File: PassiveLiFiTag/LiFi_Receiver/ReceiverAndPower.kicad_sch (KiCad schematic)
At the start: 10 parts, among them U1 TS881ILT, U3 BQ25570RGRR

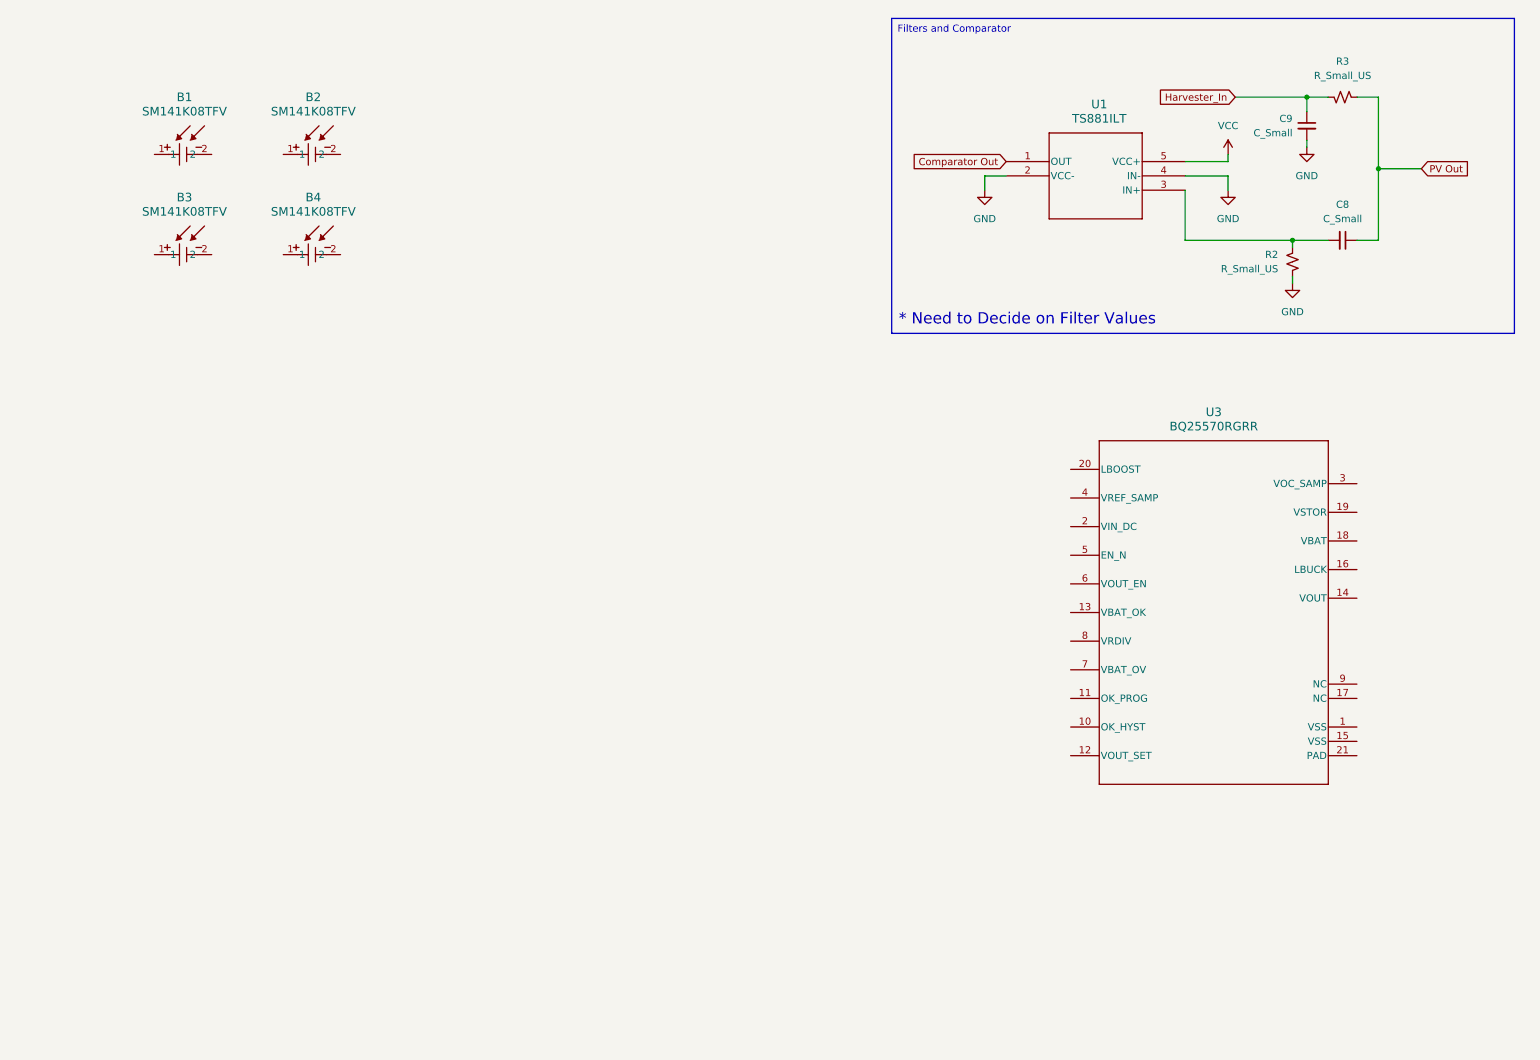
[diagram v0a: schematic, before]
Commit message: Continuing to update Hardware Design
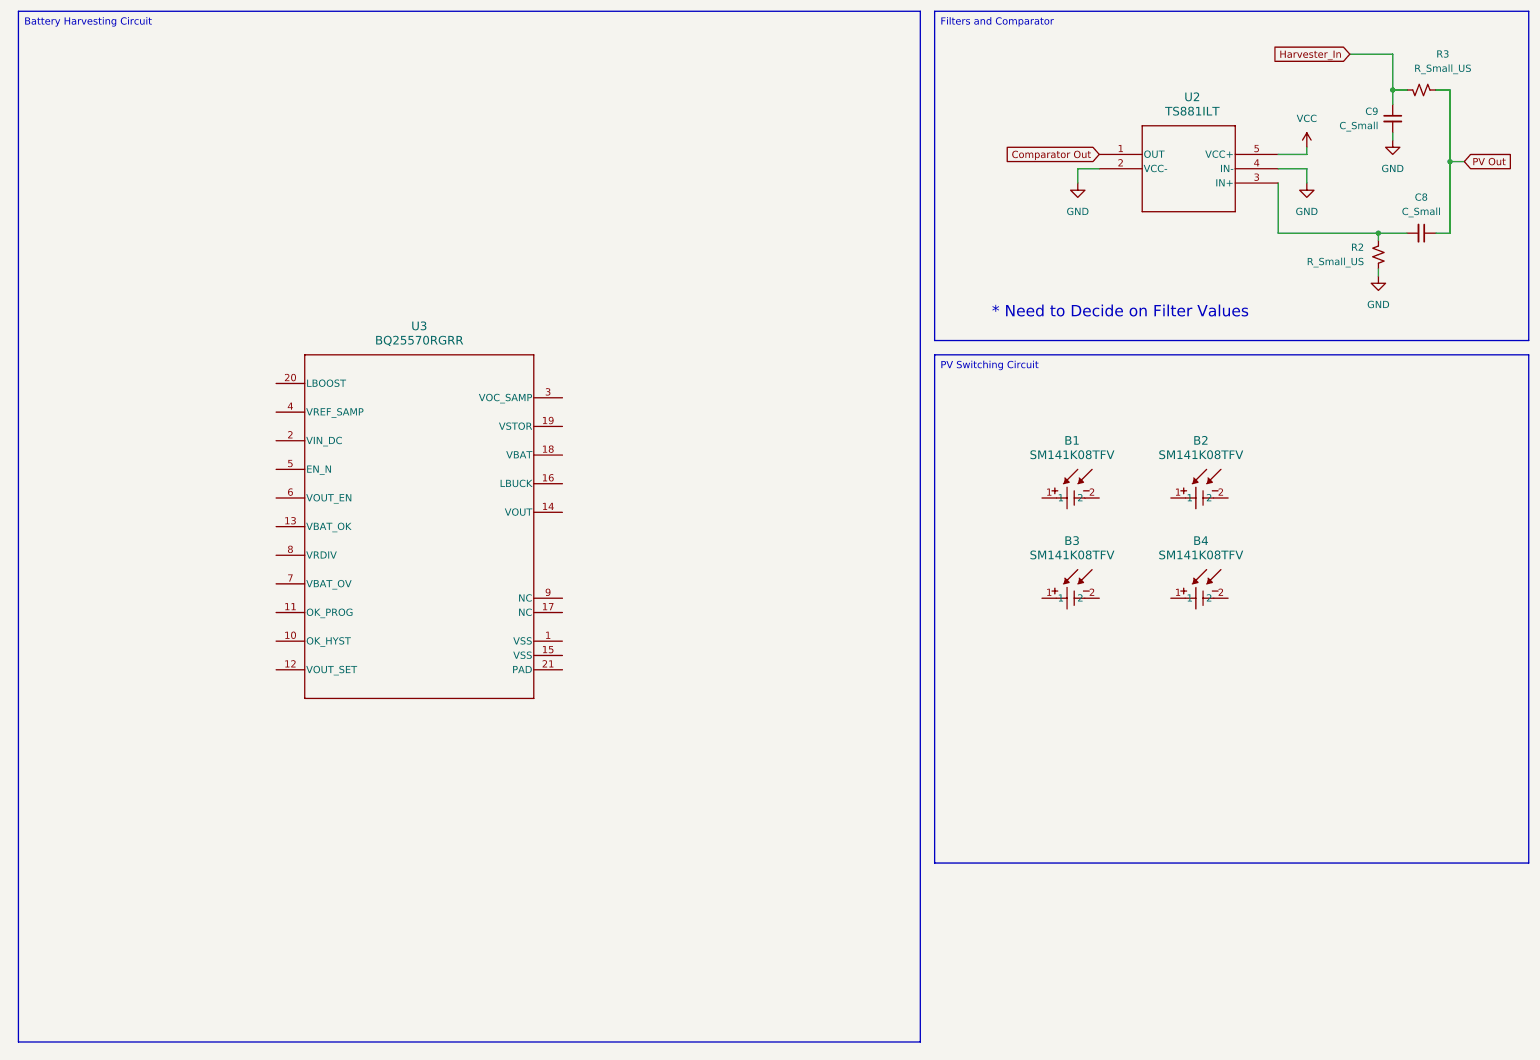
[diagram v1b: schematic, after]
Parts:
- renumbered U1 to U2
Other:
- moved on the sheet: B1, B2, B3, B4, C8, C9, R2, R3, U2, U3

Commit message: updating changes
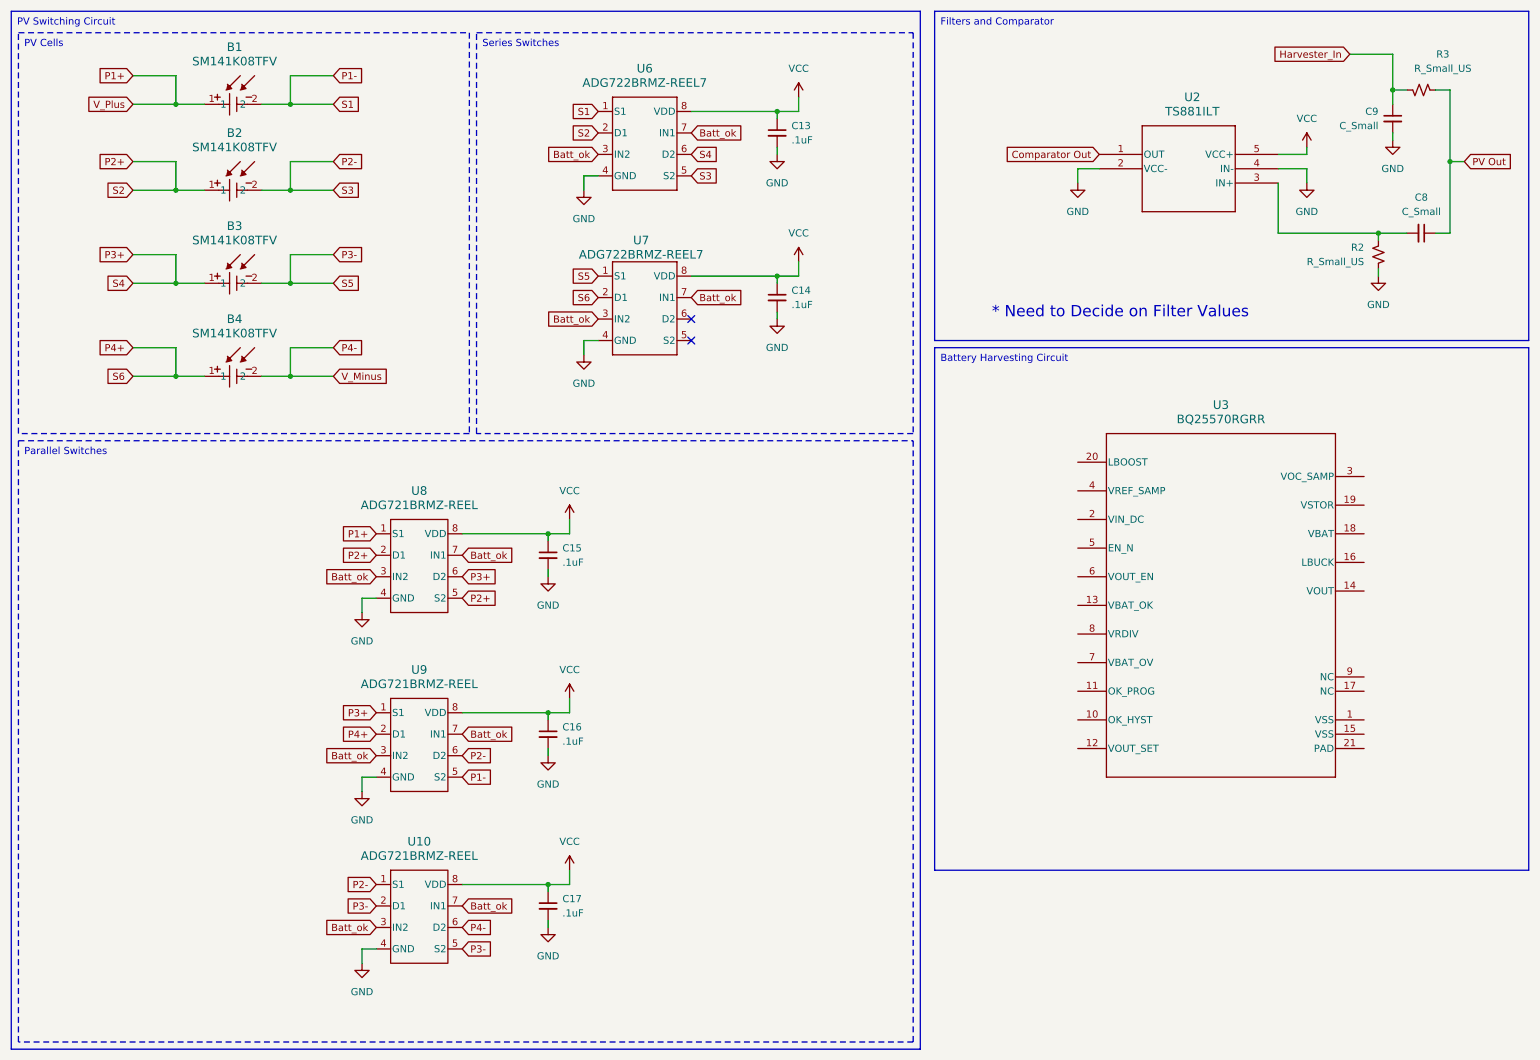
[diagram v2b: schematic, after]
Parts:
- added C13, C14, C15, C16, C17: .1uF, symbol Device:C_Small
- added U10, U8, U9: ADG721BRMZ-REEL, RM_8_ADI, symbol LiFi_Receiver:ADG721BRMZ-REEL
- added U6, U7: ADG722BRMZ-REEL7, RM_8_ADI, symbol LiFi_Receiver:ADG722BRMZ-REEL7
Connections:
- net GND: now also C13.2, C14.2, C15.2, C16.2, C17.2, U10.4 (GND), U6.4 (GND), U7.4 (GND), U8.4 (GND), U9.4 (GND)
- net VCC: now also C13.1, C14.1, C15.1, C16.1, C17.1, U10.8 (VDD), U6.8 (VDD), U7.8 (VDD), U8.8 (VDD), U9.8 (VDD)
- net P2+: now reaches B2.1
- net P2+: now also U6.2 (D1), U8.2 (D1), U8.5 (S2)
- net P2-: now reaches B2.2
- net P2-: now also U10.1 (S1), U6.5 (S2), U9.6 (D2)
- net P3+: now reaches B3.1
- net P3+: now also U6.6 (D2), U8.6 (D2), U9.1 (S1)
- net P3-: now reaches B3.2
- net P3-: now also U10.2 (D1), U10.5 (S2), U7.1 (S1)
- net P1+: now reaches B1.1
- net P1+: now also U8.1 (S1)
- net P1-: now reaches B1.2
- net P1-: now also U6.1 (S1), U9.5 (S2)
- net P4+: now reaches B4.1
- net P4+: now also U7.2 (D1), U9.2 (D1)
- net P4-: now reaches B4.2
- net P4-: now also U10.6 (D2)
- new net Batt_ok: U10.3 (IN2), U10.7 (IN1), U6.3 (IN2), U6.7 (IN1), U7.3 (IN2), U7.7 (IN1), U8.3 (IN2), U8.7 (IN1), U9.3 (IN2), U9.7 (IN1)
- no-connect marks 0 -> 2
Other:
- moved on the sheet: B1, B2, B3, B4, U3

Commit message: added Updates
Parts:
- C13, C14, C15, C16, C17: footprint (none) -> Capacitor_SMD:C_01005_0402Metric
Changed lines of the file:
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@@
       (effects (font (size 1.27 1.27)) (justify right))
     )
-    (property "Footprint" "" (at 149.86 34.29 0)
+    (property "Footprint" "Capacitor_SMD:C_01005_0402Metric" (at 149.86 34.29 0)
       (effects (font (size 1.27 1.27)) hide)
     )
@@
       (effects (font (size 1.27 1.27)) (justify right))
     )
-    (property "Footprint" "" (at 109.22 109.22 0)
+    (property "Footprint" "Capacitor_SMD:C_01005_0402Metric" (at 109.22 109.22 0)
       (effects (font (size 1.27 1.27)) hide)
     )
@@
       (effects (font (size 1.27 1.27)) (justify right))
     )
-    (property "Footprint" "" (at 149.86 63.5 0)
+    (property "Footprint" "Capacitor_SMD:C_01005_0402Metric" (at 149.86 63.5 0)
       (effects (font (size 1.27 1.27)) hide)
     )
@@
       (effects (font (size 1.27 1.27)) (justify right))
     )
-    (property "Footprint" "" (at 109.22 171.45 0)
+    (property "Footprint" "Capacitor_SMD:C_01005_0402Metric" (at 109.22 171.45 0)
       (effects (font (size 1.27 1.27)) hide)
     )
@@
       (effects (font (size 1.27 1.27)) (justify right))
     )
-    (property "Footprint" "" (at 109.22 140.97 0)
-      (effects (font (size 1.27 1.27)) hide)
-    )
+    (property "Footprint" "Capacitor_SMD:C_01005_0402Metric" (at 109.22 140.97 0)
+      (effects (font (size 1.27 1.27)) hide)
+    )
